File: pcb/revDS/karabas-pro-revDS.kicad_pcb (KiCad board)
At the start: 2 copper layers, 101.6 x 147.3 mm, 215 parts, among them CON1 CF-CARD, CON2 SD, CON3 VGA, CON4 Joystick, CON5 Keyboard, CON6 Mouse, CON7 Audio, CON8 12V, CON9 MicroSD', J1 Floppy, J10 Ext Joystick, J2 FPGA JTAG, J3 Floppy, J4 uBus, J5 AVR JTAG, J6 AVR UART, J7 ESP-BUS, J8 Tape In, J9 Tape Out, Q1 BC856, Q2 BC548, SW1 SW_Push, SW2 SW_Push, SW4 SW_SPST, U1 EP4CE10E22C8N, U10 ESP-12E, U11 TDA1543, U12 AMS1117-3.3, U13 AMS1117-2.5, U14 AMS1117-1.2, U15 LM2596S-5, U16 LM311, U17 74LS06, U18 74LS38, U2 CY62167EV30LL, U3 W25Q16, U3''1 W25Q16, U4 EPM3128ATC100-10N, U5 ATMEGA328-AU, U6 MB8877A, U7 TXB0104PW, U8 TXB0104PW, U9 DS1307Z+, X1 SG-7050CAN, Y1 32768Hz, Y2 16MHz

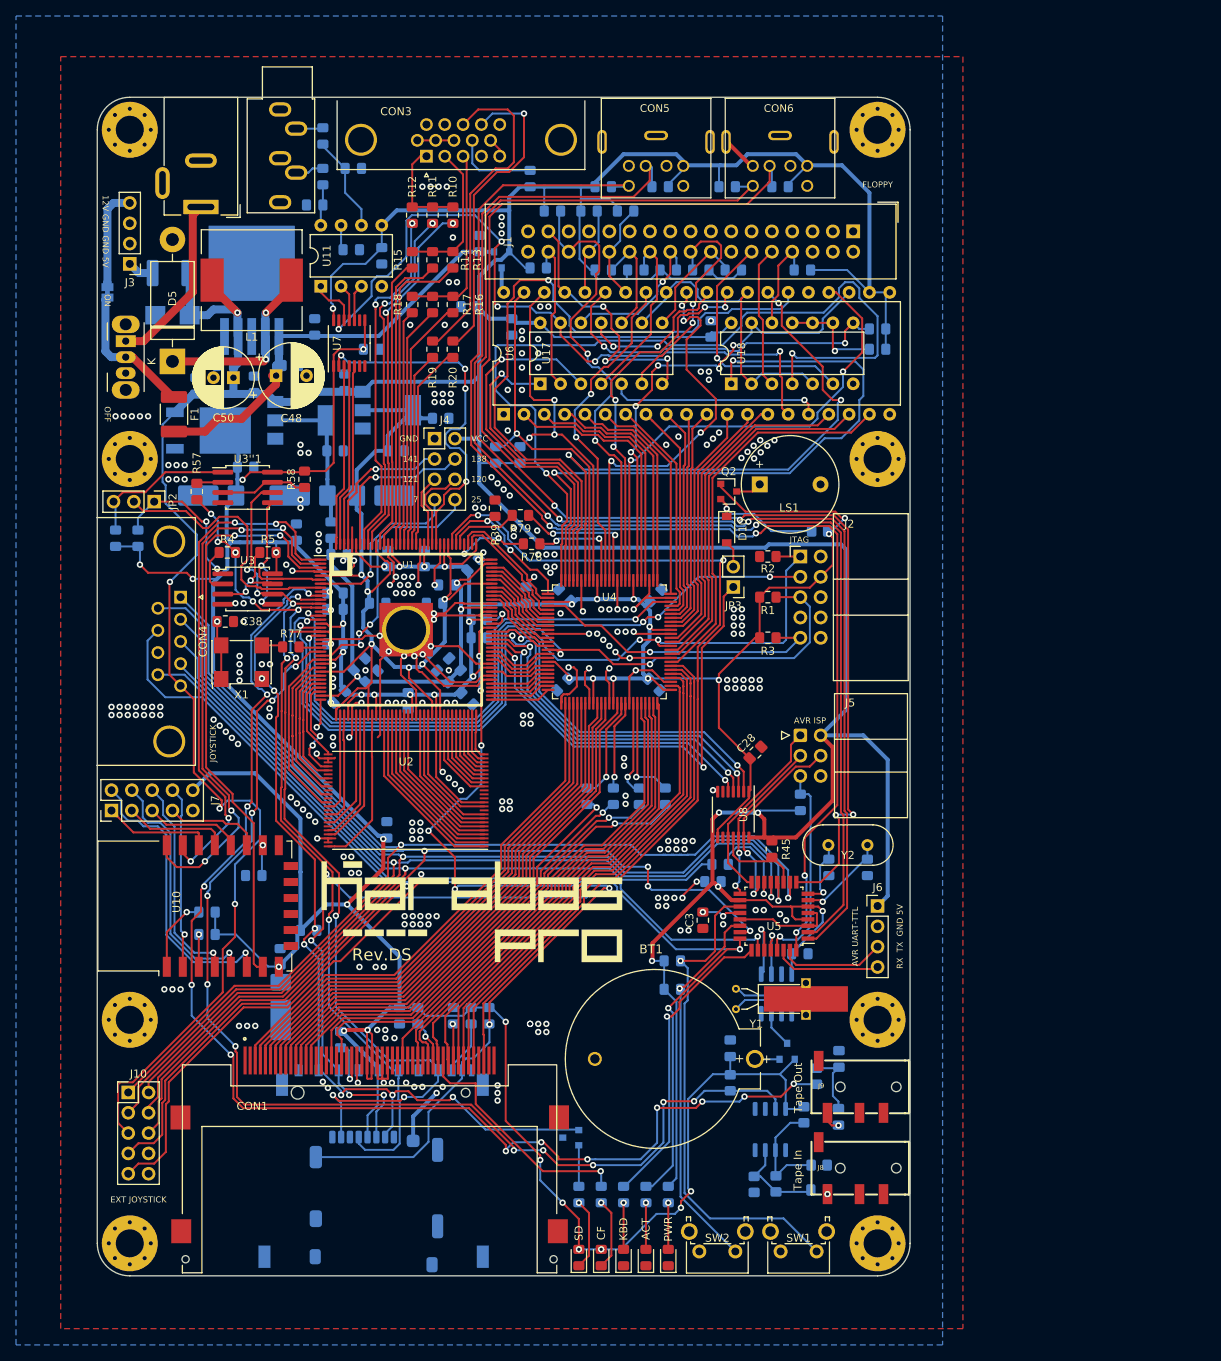
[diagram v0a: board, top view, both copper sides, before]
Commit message: latest version
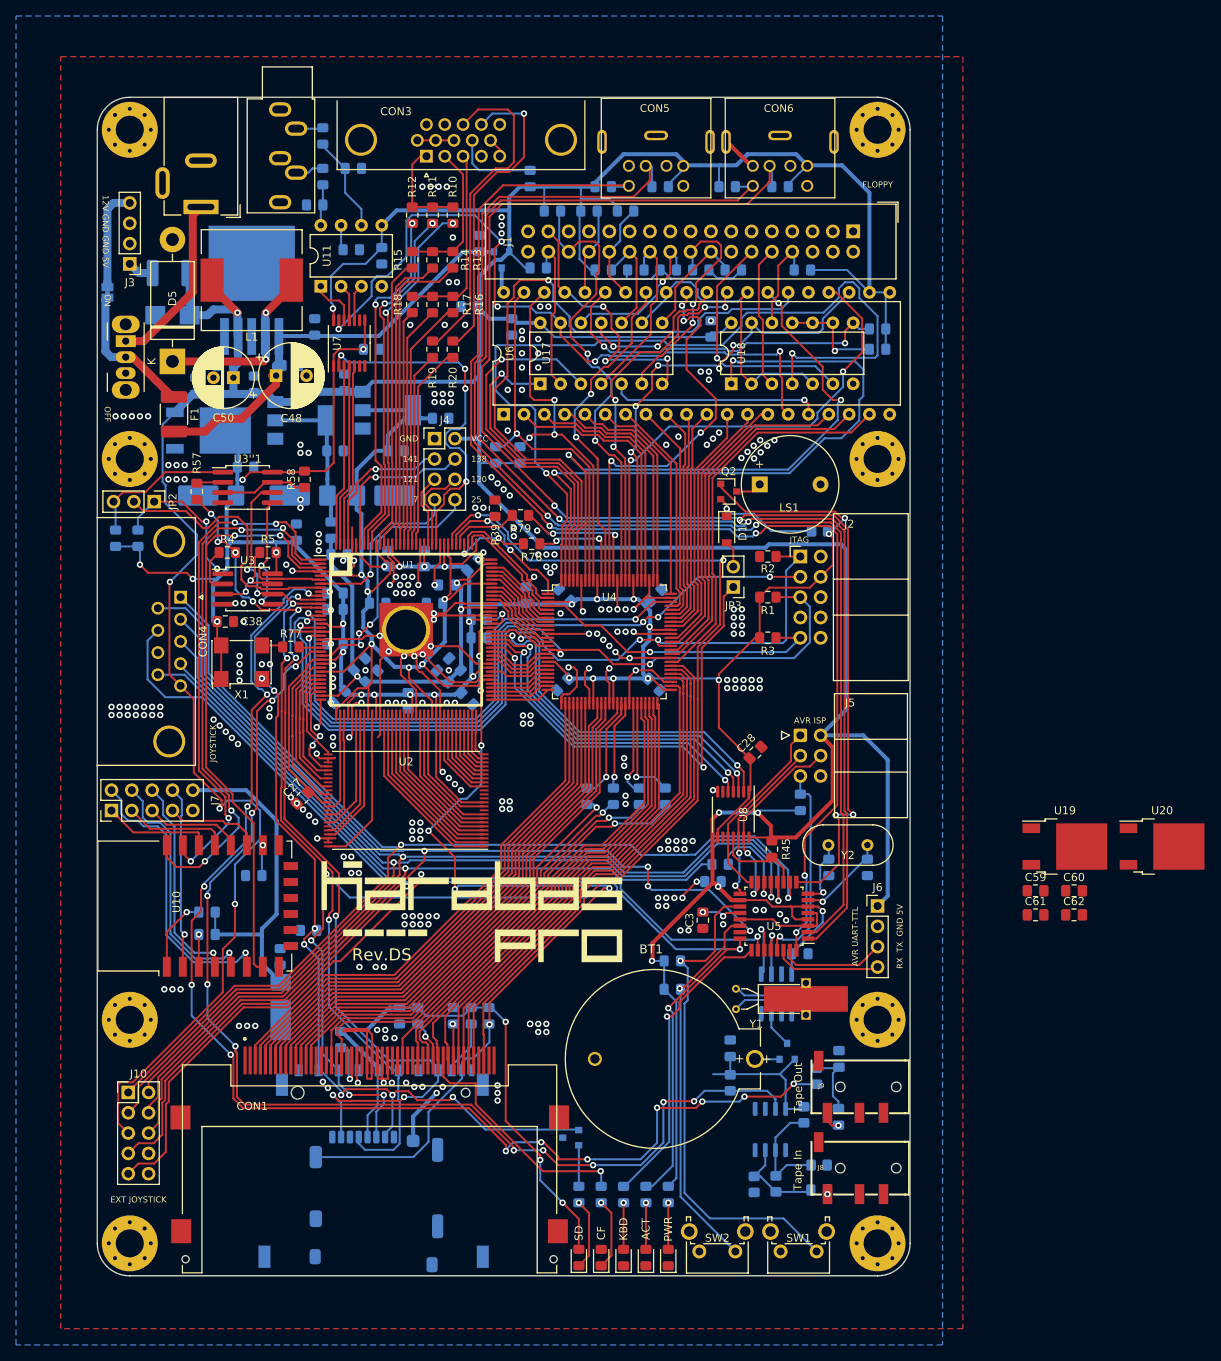
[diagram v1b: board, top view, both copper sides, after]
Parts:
- added C59: 1uF, Capacitor_SMD:C_0805_2012Metric_Pad1.18x1.45mm_HandSolder, F.Cu at (216.3, 124.6)
- added C60: 1uF, Capacitor_SMD:C_0805_2012Metric_Pad1.18x1.45mm_HandSolder, F.Cu at (221.2, 124.6)
- added C61: 1uF, Capacitor_SMD:C_0805_2012Metric_Pad1.18x1.45mm_HandSolder, F.Cu at (216.3, 127.6)
- added C62: 1uF, Capacitor_SMD:C_0805_2012Metric_Pad1.18x1.45mm_HandSolder, F.Cu at (221.2, 127.6)
- added U19: AMS1117-3.3, Package_TO_SOT_SMD:TO-252-2, F.Cu at (220.0, 119.1)
- added U20: AMS1117-3.3, Package_TO_SOT_SMD:TO-252-2, F.Cu at (232.2, 119.1)
- C27: moved to F.Cu
- moved C27 11.3 mm to (124.7, 113.0), turned to 225 degrees
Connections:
- C13 pad 1: VCC3_3 -> /+3.3ESP
- C18 pad 1: VCC3_3 -> /+3.3ESP
- C54 pad 1: VCC3_3 -> /+3.3ESP
- CON1 pad 13: VCC3_3 -> +3.3VP
- CON1 pad 38: VCC3_3 -> +3.3VP
- CON2 pad 4: VCC3_3 -> +3.3VP
- CON9 pad 4: VCC3_3 -> +3.3VP
- D4 pad 2: VCC3_3 -> +3.3VP
- D6 pad 2: VCC3_3 -> +3.3VP
- J7 pad 10: VCC3_3 -> /+3.3ESP
- R30 pad 2: VCC3_3 -> /+3.3ESP
- R31 pad 2: VCC3_3 -> /+3.3ESP
- R36 pad 2: VCC3_3 -> +3.3VP
- R37 pad 1: VCC3_3 -> +3.3VP
- R52 pad 2: VCC3_3 -> +3.3VP
- R74 pad 1: VCC3_3 -> +3.3VP
- R75 pad 1: VCC3_3 -> +3.3VP
- U10 pad 8: VCC3_3 -> /+3.3ESP
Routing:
- net VCC3_3: track 642.5 -> 405.1 mm, vias 41 -> 29
- net +3.3VP: track 0.00 -> 84.5 mm, vias 0 -> 3
- net /+3.3ESP: track 0.00 -> 45.1 mm
- net VCC: track 650.9 -> 651.4 mm

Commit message: Revert "latest version"
This reverts commit fe14166d25968ab133076a7a9191b22261ce910e.
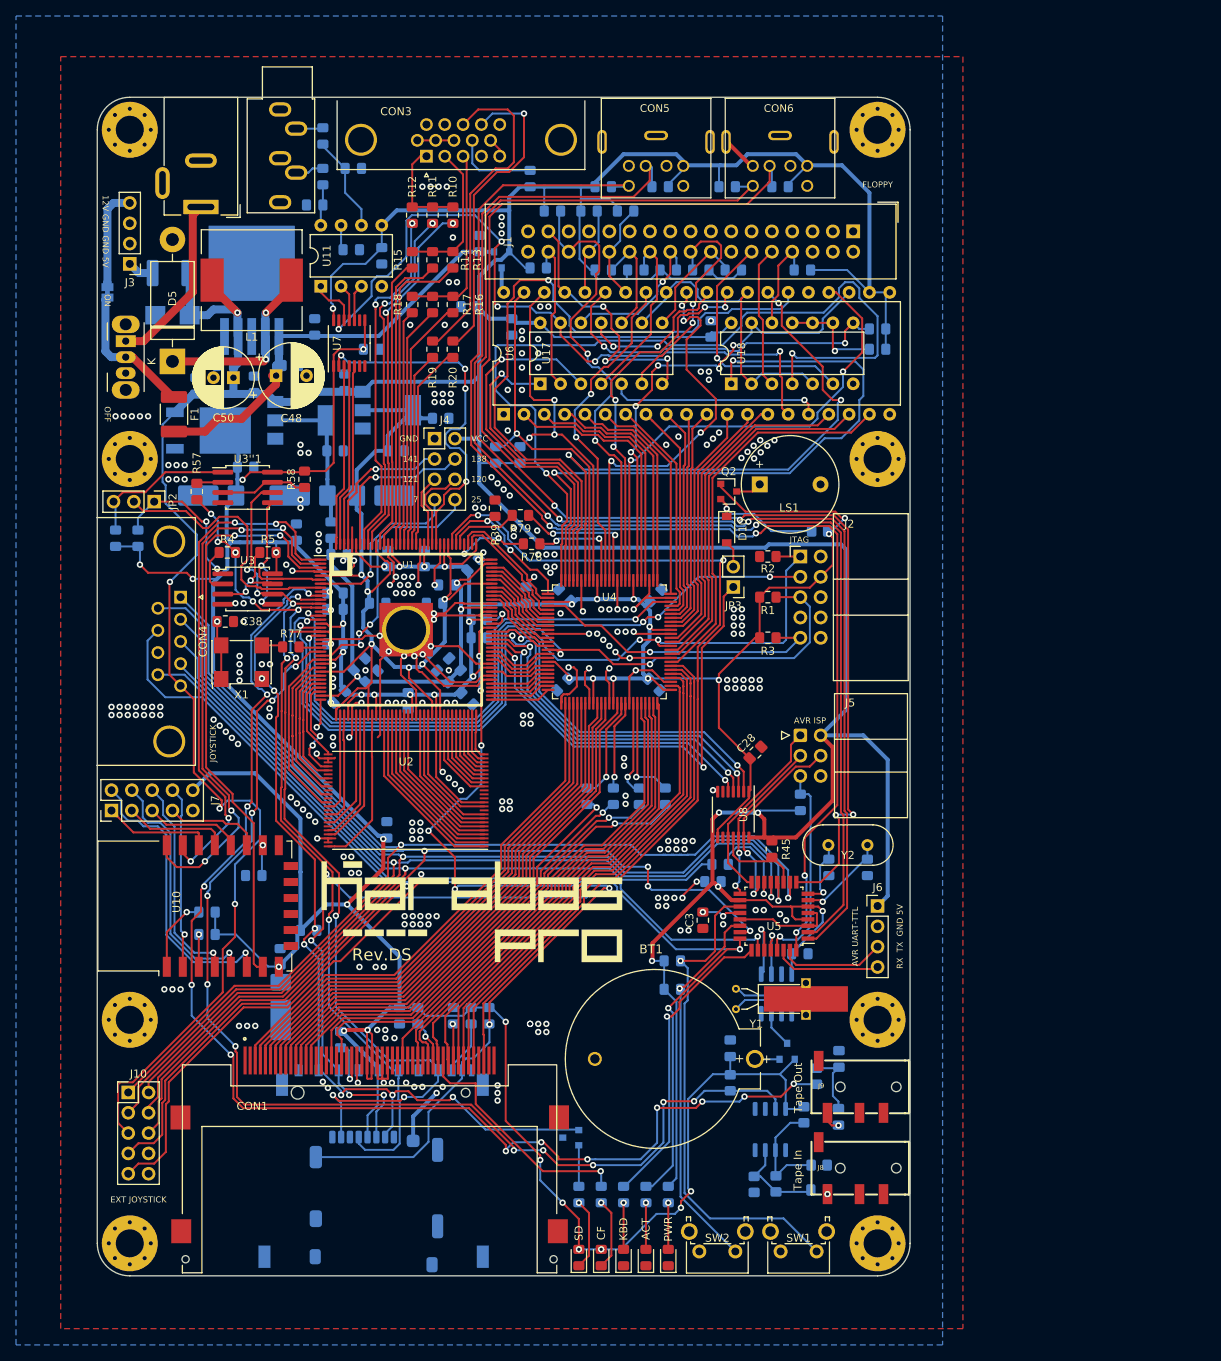
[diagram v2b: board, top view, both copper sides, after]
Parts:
- removed C59, C60, C61, C62: 1uF, Capacitor_SMD:C_0805_2012Metric_Pad1.18x1.45mm_HandSolder
- removed U19, U20: AMS1117-3.3, Package_TO_SOT_SMD:TO-252-2
- C27: moved to B.Cu
- moved C27 11.3 mm to (135.3, 117.0), turned to 90 degrees
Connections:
- C13 pad 1: /+3.3ESP -> VCC3_3
- C18 pad 1: /+3.3ESP -> VCC3_3
- C54 pad 1: /+3.3ESP -> VCC3_3
- CON1 pad 13: +3.3VP -> VCC3_3
- CON1 pad 38: +3.3VP -> VCC3_3
- CON2 pad 4: +3.3VP -> VCC3_3
- CON9 pad 4: +3.3VP -> VCC3_3
- D4 pad 2: +3.3VP -> VCC3_3
- D6 pad 2: +3.3VP -> VCC3_3
- J7 pad 10: /+3.3ESP -> VCC3_3
- R30 pad 2: /+3.3ESP -> VCC3_3
- R31 pad 2: /+3.3ESP -> VCC3_3
- R36 pad 2: +3.3VP -> VCC3_3
- R37 pad 1: +3.3VP -> VCC3_3
- R52 pad 2: +3.3VP -> VCC3_3
- R74 pad 1: +3.3VP -> VCC3_3
- R75 pad 1: +3.3VP -> VCC3_3
- U10 pad 8: /+3.3ESP -> VCC3_3
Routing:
- net VCC3_3: track 405.1 -> 642.5 mm, vias 29 -> 41
- net +3.3VP: track 84.5 -> 0.00 mm, vias 3 -> 0
- net /+3.3ESP: track 45.1 -> 0.00 mm
- net VCC: track 651.4 -> 650.9 mm
